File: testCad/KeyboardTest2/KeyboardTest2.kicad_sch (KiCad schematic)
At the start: 44 parts, among them J1 Conn_02x12_Top_Bottom, J2 AudioJack4

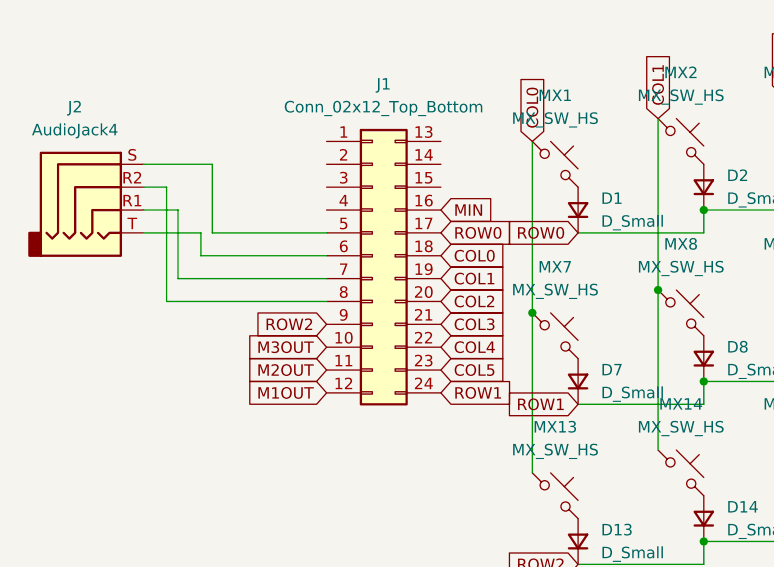
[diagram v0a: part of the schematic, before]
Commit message: 3D cad and pcb layout
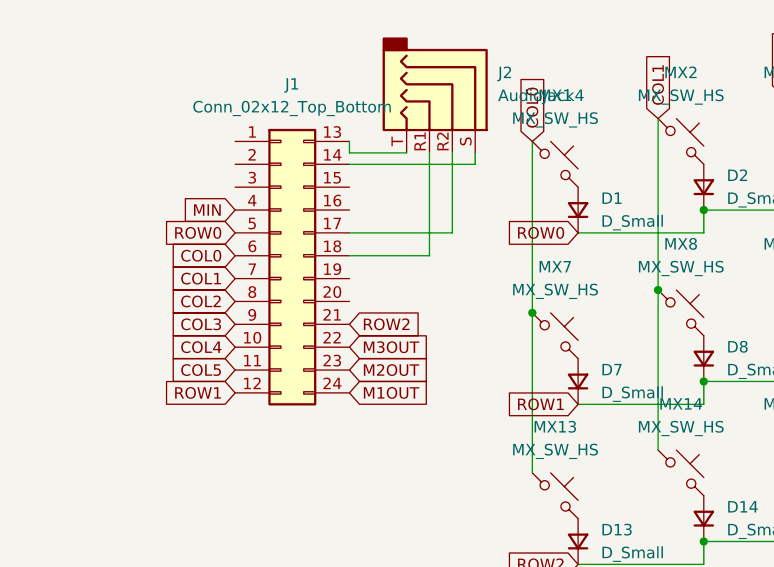
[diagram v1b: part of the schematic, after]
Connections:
- net COL0: now also J1.6 (Pin_6); no longer J1.18 (Pin_18)
- net COL1: now also J1.7 (Pin_7); no longer J1.19 (Pin_19)
- net COL2: now also J1.8 (Pin_8); no longer J1.20 (Pin_20)
- net COL3: now also J1.9 (Pin_9); no longer J1.21 (Pin_21)
- net COL4: now also J1.10 (Pin_10); no longer J1.22 (Pin_22)
- net COL5: now also J1.11 (Pin_11); no longer J1.23 (Pin_23)
- net M1OUT: now also J1.24 (Pin_24); no longer J1.12 (Pin_12)
- net M2OUT: now also J1.23 (Pin_23); no longer J1.11 (Pin_11)
- net M3OUT: now also J1.22 (Pin_22); no longer J1.10 (Pin_10)
- net MIN: now also J1.4 (Pin_4); no longer J1.16 (Pin_16)
- net ROW0: now also J1.5 (Pin_5); no longer J1.17 (Pin_17)
- net ROW1: now also J1.12 (Pin_12); no longer J1.24 (Pin_24)
- net ROW2: now also J1.21 (Pin_21); no longer J1.9 (Pin_9)
- net at J1.13 (Pin_13): now also J2.T
- net at J1.14 (Pin_14): now also J2.S
- net at J2.R1: now also J1.18 (Pin_18); no longer J1.7 (Pin_7)
- net at J2.R2: now also J1.17 (Pin_17); no longer J1.8 (Pin_8)
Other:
- moved on the sheet: J1, J2
